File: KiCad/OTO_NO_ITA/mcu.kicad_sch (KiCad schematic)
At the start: 1 part, among them U1 STM32H7S3Z8Tx

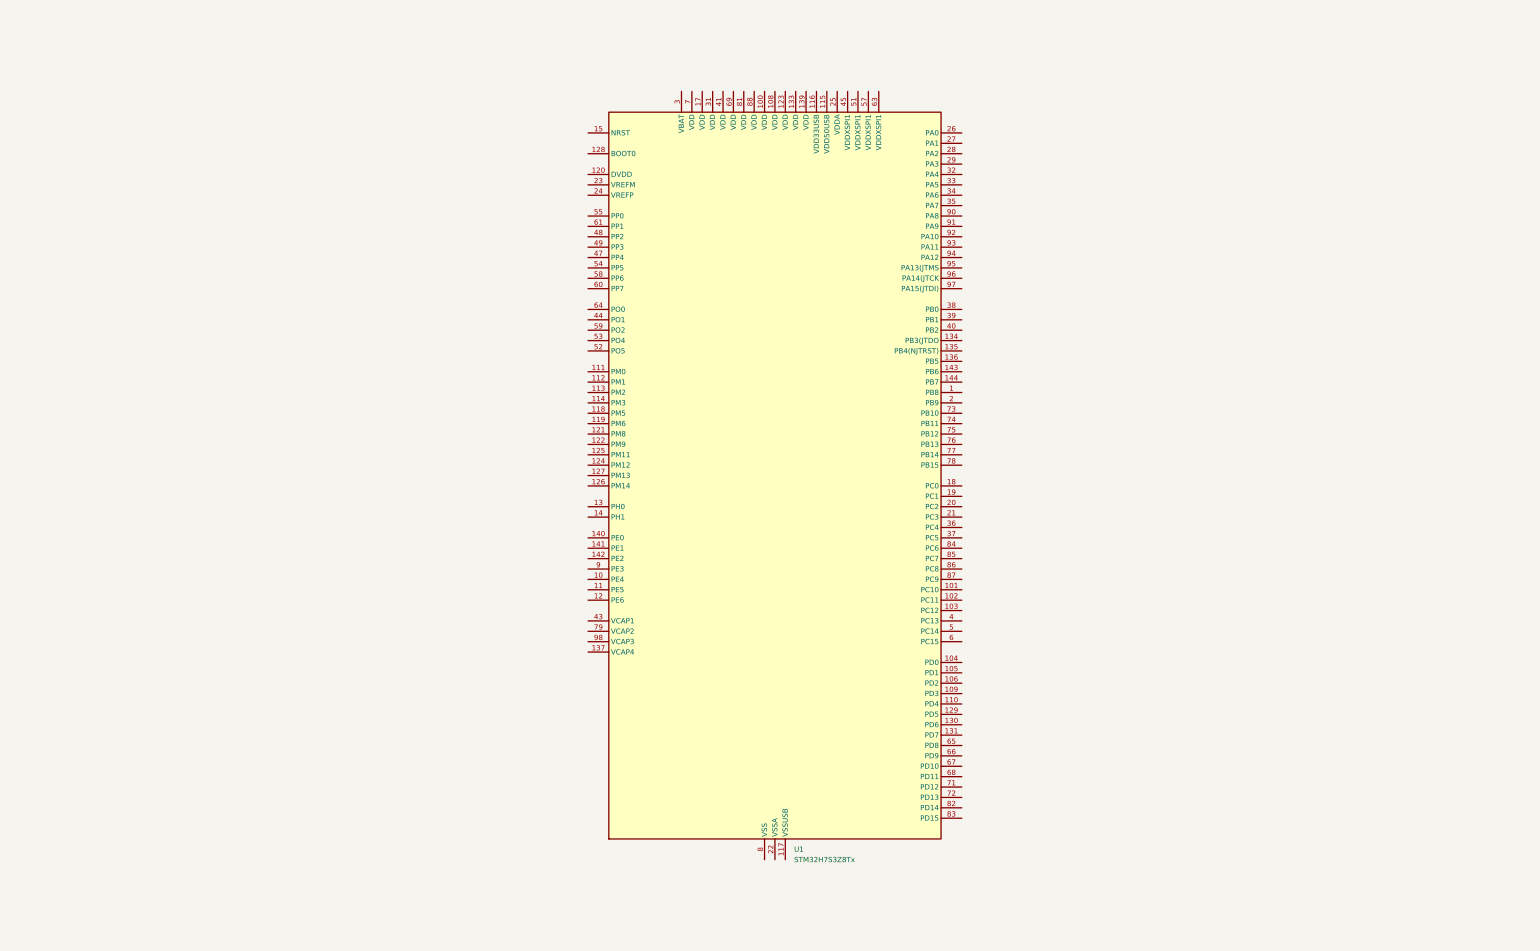
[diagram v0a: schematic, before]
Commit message: Updated schematics.
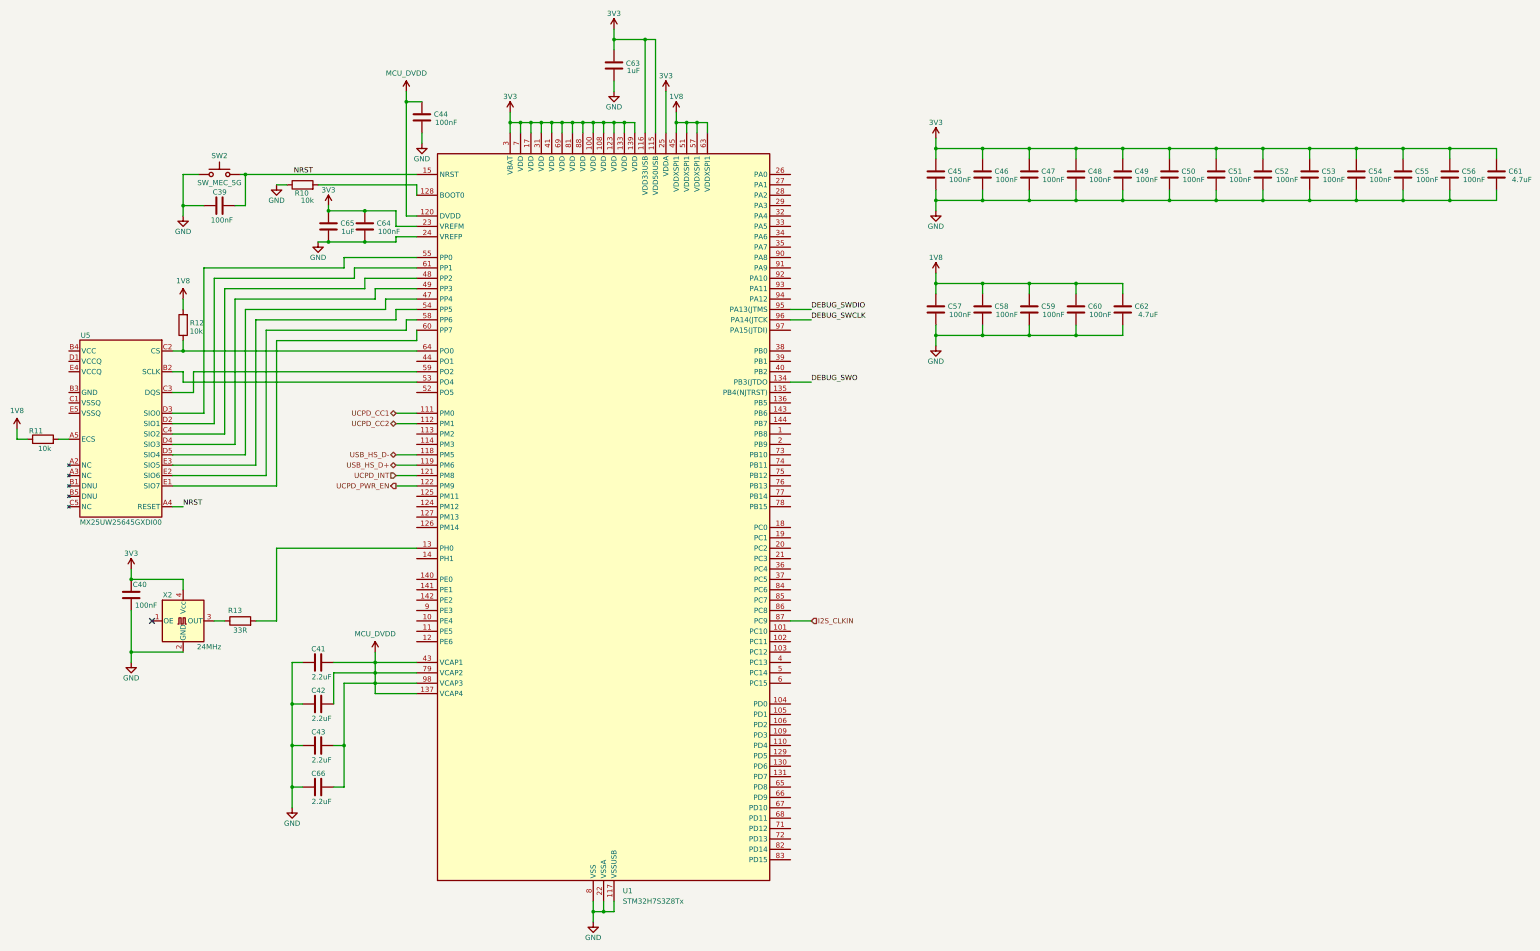
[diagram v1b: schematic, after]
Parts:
- added C39, C44, C45, C46, C47, C48, C49, C50, C51, C52, C53, C54, C55, C56, C57, C58, C59, C60, C64: 100nF, symbol Device:C
- added C40: 100nF, Capacitor_SMD:C_0402_1005Metric, symbol Device:C
- added C41, C42, C43, C66: 2.2uF, symbol Device:C
- added C61, C62: 4.7uF, symbol Device:C
- added C63, C65: 1uF, symbol Device:C
- added R10, R11, R12: 10k, symbol Device:R
- added R13: 33R, Resistor_SMD:R_0402_1005Metric, symbol Device:R
- added SW2: SW_MEC_5G, symbol My_Parts:SW_MEC_5G
- added U5: MX25UW25645GXDI00, symbol My_Parts:MX25UW25645GXDI00
- added X2: 24MHz, symbol Oscillator:SG-8002CE
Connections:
- net 3V3: now reaches U1.100 (VDD)
- net 3V3: now also U1.108 (VDD), U1.115 (VDD50USB), U1.116 (VDD33USB), U1.123 (VDD), U1.133 (VDD), U1.139 (VDD), U1.17 (VDD), U1.23 (VREFM), U1.25 (VDDA), U1.3 (VBAT), U1.31 (VDD), U1.41 (VDD), U1.69 (VDD), U1.7 (VDD), U1.81 (VDD), U1.88 (VDD), C40.2, C45.2, C46.2, C47.2, C48.2, C49.2, C50.2, C51.2, C52.2, C53.2, C54.2, C55.2, C56.2, C61.2, C63.2, C64.2, C65.2, X2.4 (Vcc)
- net GND: now reaches U1.107 (VSS), U1.132 (VSS), U1.138 (VSS), U1.16 (VSS), U1.30 (VSS), U1.42 (VSS), U1.46 (VSS), U1.50 (VSS), U1.56 (VSS), U1.62 (VSS), U1.70 (VSS), U1.8 (VSS), U1.80 (VSS), U1.89 (VSS), U1.99 (VSS)
- net GND: now also U1.117 (VSSUSB), U1.22 (VSSA), U1.24 (VREFP), C39.1, C40.1, C41.1, C42.1, C43.1, C44.1, C45.1, C46.1, C47.1, C48.1, C49.1, C50.1, C51.1, C52.1, C53.1, C54.1, C55.1, C56.1, C57.1, C58.1, C59.1, C60.1, C61.1, C62.1, C63.1, C64.1, C65.1, C66.1, R10.1, SW2.1 (A), X2.2 (GND)
- net UCPD_CC1: now reaches U1.111 (PM0)
- net UCPD_CC2: now reaches U1.112 (PM1)
- net USB_HS_D-: now reaches U1.118 (PM5)
- net USB_HS_D+: now reaches U1.119 (PM6)
- net MCU_DVDD: now reaches U1.120 (DVDD)
- net MCU_DVDD: now also U1.137 (VCAP4), U1.43 (VCAP1), U1.79 (VCAP2), U1.98 (VCAP3), C41.2, C42.2, C43.2, C44.2, C66.2
- net UCPD_INT: now reaches U1.121 (PM8)
- net UCPD_PWR_EN: now reaches U1.122 (PM9)
- net at U1.128 (BOOT0): now also R10.2
- net at U1.13 (PH0): now also R13.2
- net DEBUG_SWO: now reaches U1.134 (PB3(JTDO)
- net NRST: now reaches U1.15 (NRST)
- net NRST: now also C39.2, SW2.3 (B), U5.A4 (RESET)
- net 1V8: now reaches U1.45 (VDDXSPI1)
- net 1V8: now also U1.51 (VDDXSPI1), U1.57 (VDDXSPI1), U1.63 (VDDXSPI1), C57.2, C58.2, C59.2, C60.2, C62.2, R11.1, R12.2
- net at U1.47 (PP4): now also U5.D5 (SIO4)
- net at U1.48 (PP2): now also U5.C4 (SIO2)
- net at U1.49 (PP3): now also U5.D4 (SIO3)
- net at U1.53 (PO4): now also U5.B2 (SCLK)
- net at U1.54 (PP5): now also U5.E3 (SIO5)
- net at U1.55 (PP0): now also U5.D3 (SIO0)
- net at U1.58 (PP6): now also U5.E2 (SIO6)
- net at U1.59 (PO2): now also U5.C3 (DQS)
- net at U1.60 (PP7): now also U5.E1 (SIO7)
- net at U1.61 (PP1): now also U5.D2 (SIO1)
- net at U1.64 (PO0): now also R12.1, U5.C2 (CS)
- net I2S_CLKIN: now reaches U1.87 (PC9)
- net DEBUG_SWDIO: now reaches U1.95 (PA13(JTMS)
- net DEBUG_SWCLK: now reaches U1.96 (PA14(JTCK)
- new net: R13.1, X2.3 (OUT)
- new net: R11.2, U5.A5 (ECS)
- no-connect marks 0 -> 1
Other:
- moved on the sheet: U1
